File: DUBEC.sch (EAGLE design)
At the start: 47 parts

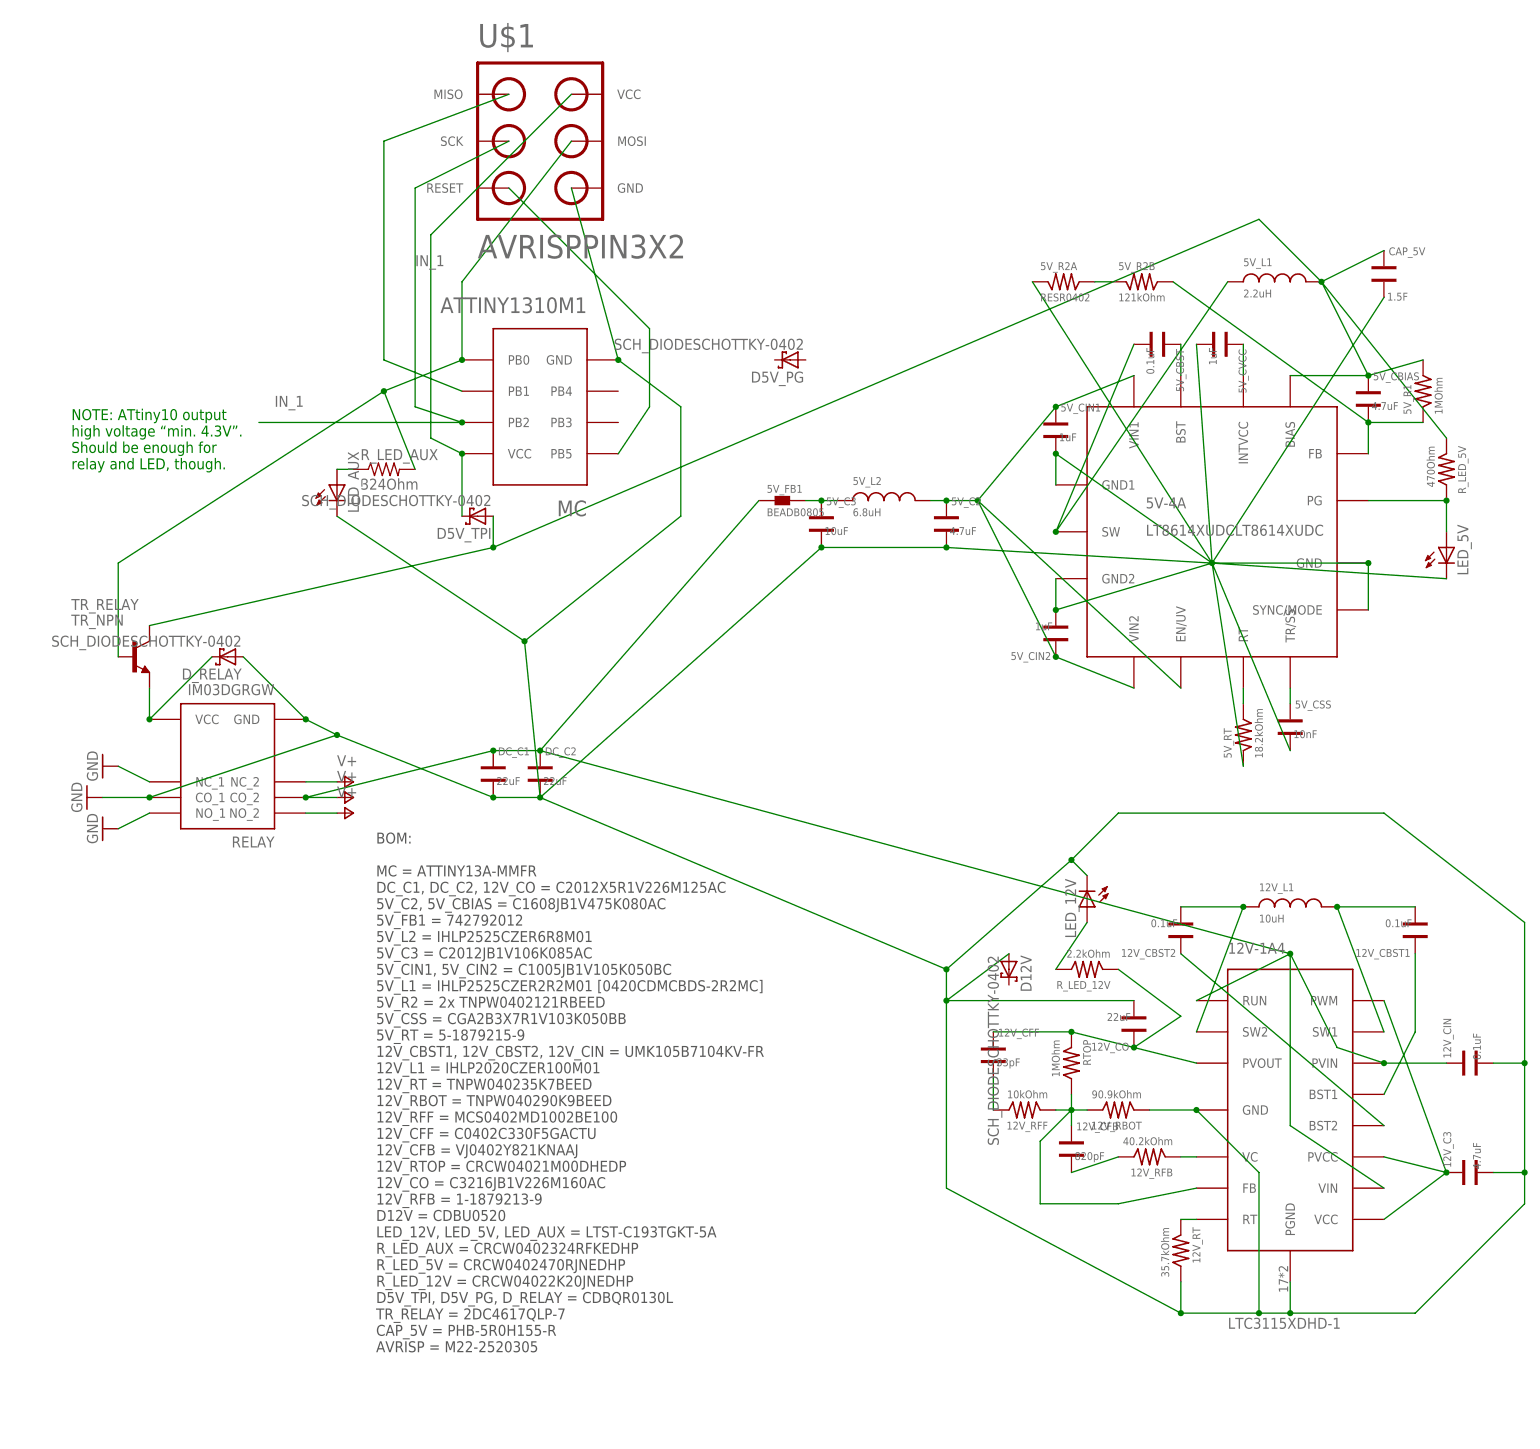
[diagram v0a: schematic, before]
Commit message: Voltage divider
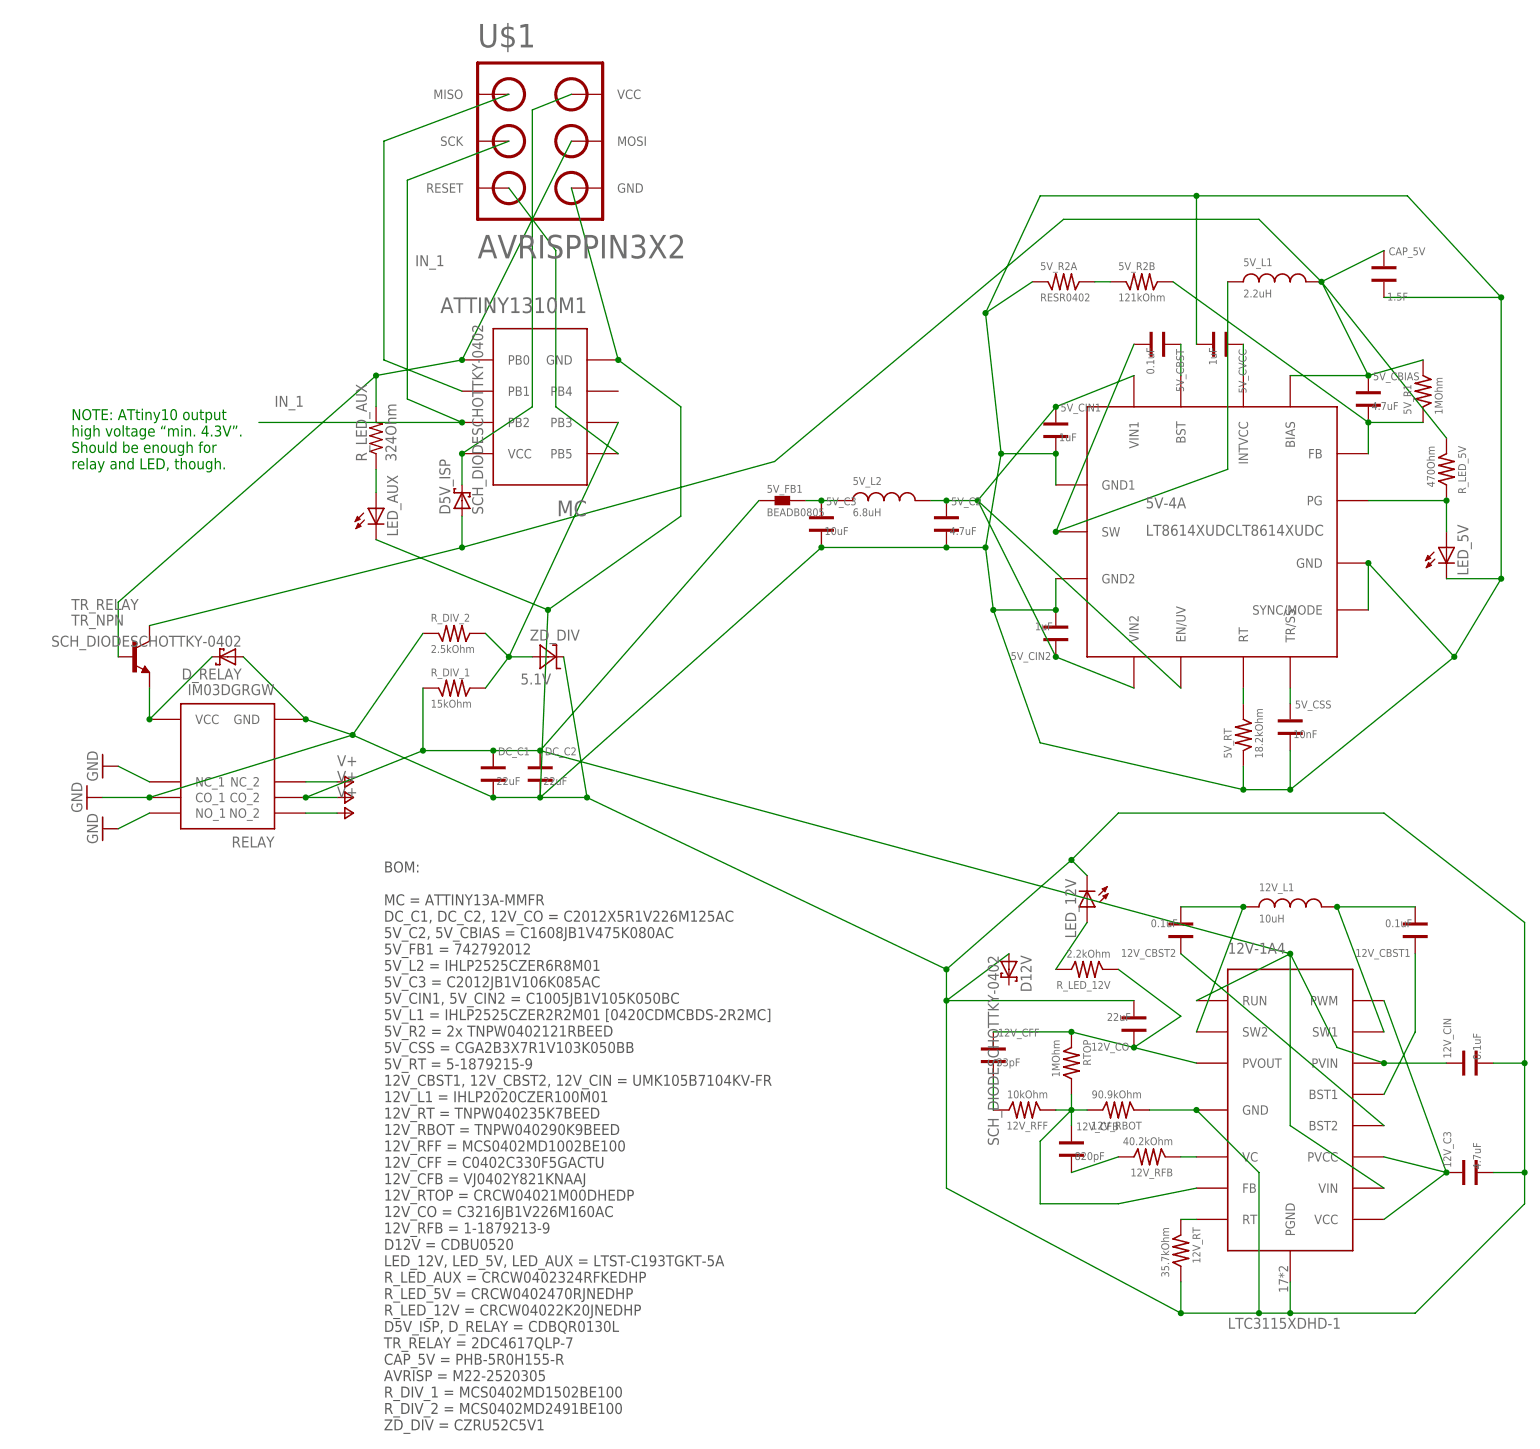
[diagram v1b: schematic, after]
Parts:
- removed D5V_PG, D5V_TPI: SCH_DIODESCHOTTKY-0402, dubec:SCH_DIODESCHOTTKY-0402
- added D5V_ISP: SCH_DIODESCHOTTKY-0402, dubec:SCH_DIODESCHOTTKY-0402
- added R_DIV_1: 15kOhm, dubec:RESR0402
- added R_DIV_2: 2.5kOhm, dubec:RESR0402
- added ZD_DIV: 5.1V, dubec:Z-DIODE
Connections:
- net N$11 renamed PB5
- net N$16 renamed MISO
- net PB0 renamed RELAY_CONTROL
- new net N$17: MC.PB3, R_DIV_1.GND, R_DIV_2.GND, ZD_DIV.A
- net 35V: now also R_DIV_1.1
- net 5V: now also D5V_ISP.A; no longer D5V_TPI.A
- net 5V_ISP: now also D5V_ISP.C; no longer D5V_TPI.C
- net GND: now also R_DIV_2.1, ZD_DIV.C
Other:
- moved on the sheet: LED_AUX, R_LED_AUX
